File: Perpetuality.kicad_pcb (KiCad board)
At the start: 2 copper layers, 33 x 36.5 mm, 27 parts, among them J1 Conn_01x04, J2 Conn_01x01, J3 Conn_01x01, J4 Conn_01x01, U1 XIAO-nRF52840-SMD, U2 NCV8164CSN180T1G, U3 ICM-20948, U4 INA333xxDGK, U5 OPA333xxDCK, U6 ADS8866IDGS

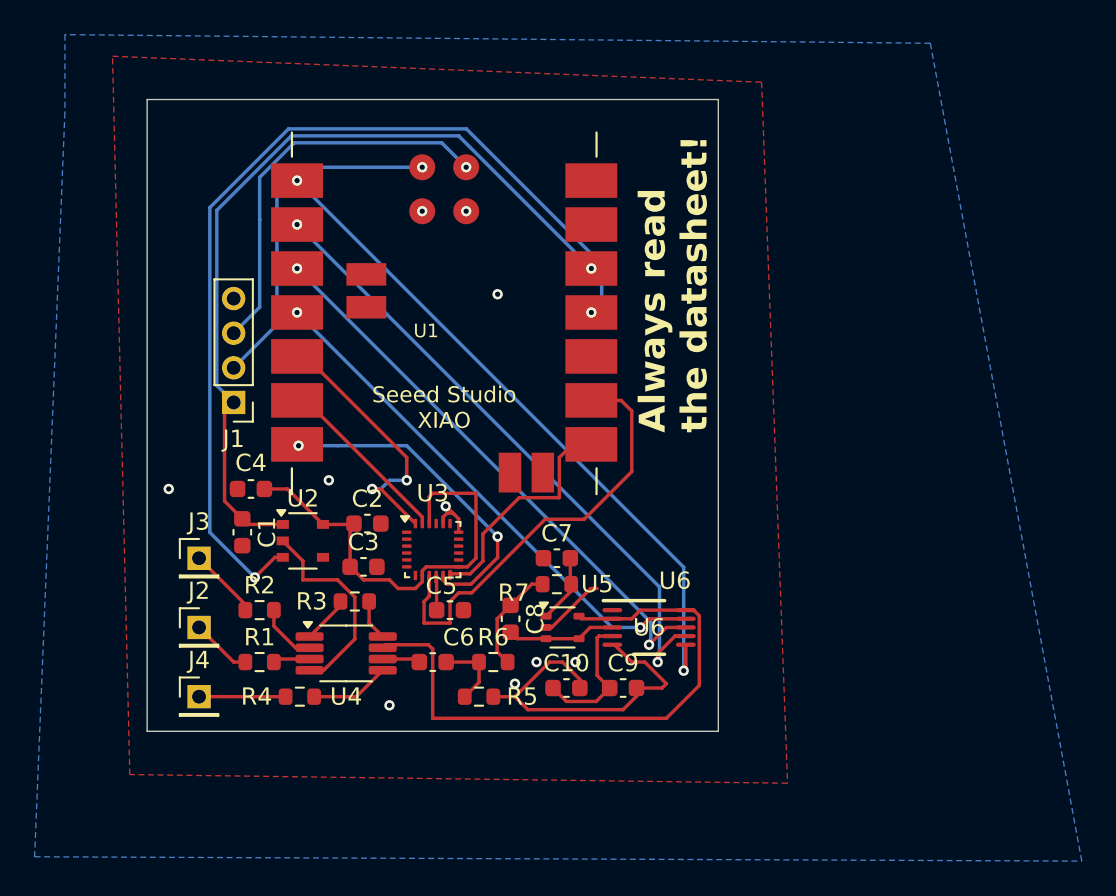
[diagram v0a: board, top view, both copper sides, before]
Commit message: newest version sent to jlc
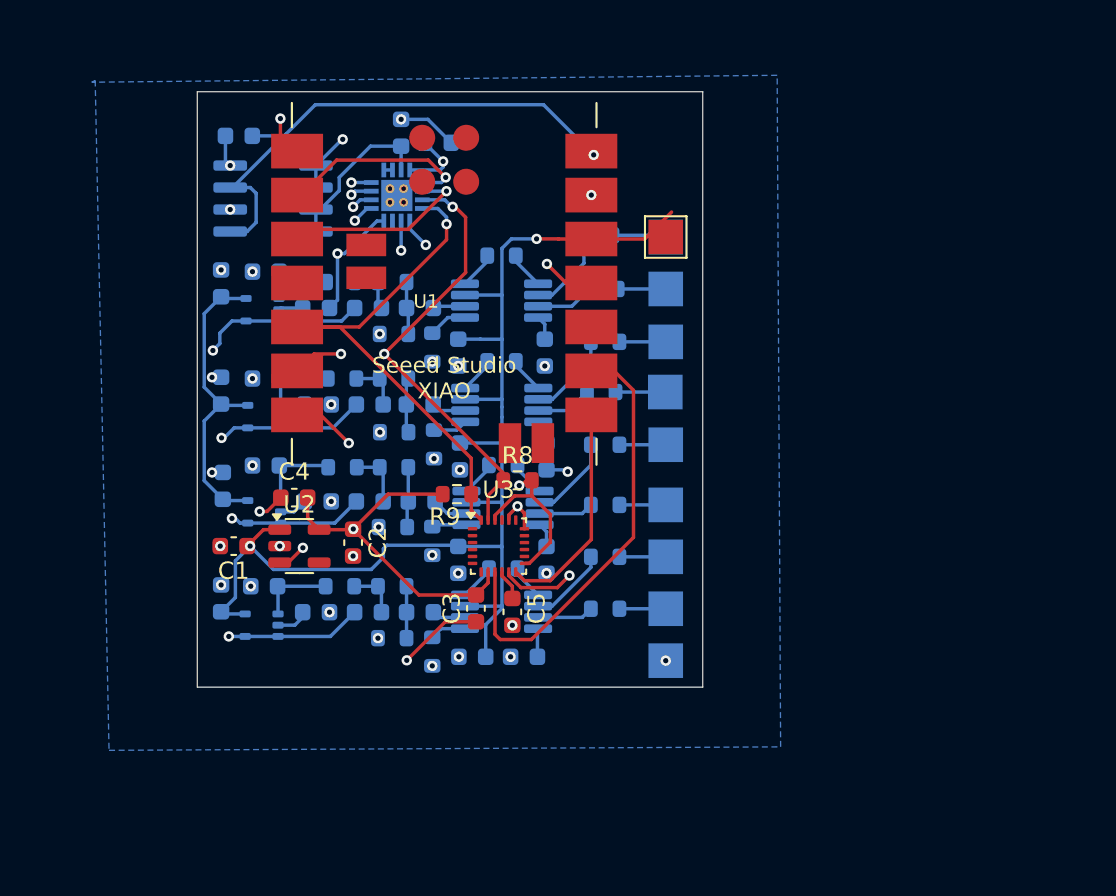
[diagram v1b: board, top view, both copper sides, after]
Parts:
- added ...: Conn_01x01, TestPoint:TestPoint_Pad_2.0x2.0mm, B.Cu at (80.5, 78.0)
- added C11: 33nF, Capacitor_SMD:C_0603_1608Metric, B.Cu at (63.4, 81.6)
- added C12: 33nF, Capacitor_SMD:C_0603_1608Metric, B.Cu at (57.4, 80.1)
- added C13: 0.1uF, Capacitor_SMD:C_0603_1608Metric, B.Cu at (60.4, 81.6)
- added C14: 0.1uF, Capacitor_SMD:C_0603_1608Metric, B.Cu at (54.8, 80.8)
- added C15: 2.2µF, Capacitor_SMD:C_0603_1608Metric, B.Cu at (55.8, 66.1)
- added C16: 1µF, Capacitor_SMD:C_0603_1608Metric, B.Cu at (66.3, 76.0)
- added C17: 0.1uF, Capacitor_SMD:C_0603_1608Metric, B.Cu at (73.5, 78.6)
- added C18: 0.1uF, Capacitor_SMD:C_0603_1608Metric, B.Cu at (68.5, 78.6)
- added C19: 33nF, Capacitor_SMD:C_0603_1608Metric, B.Cu at (57.4, 73.9)
- added C20: 33nF, Capacitor_SMD:C_0603_1608Metric, B.Cu at (63.3, 76.0)
- added C21: 0.1uF, Capacitor_SMD:C_0603_1608Metric, B.Cu at (60.3, 76.0)
- added C22: 0.1uF, Capacitor_SMD:C_0603_1608Metric, B.Cu at (54.8, 74.6)
- added C23: 0.1uF, Capacitor_SMD:C_0603_1608Metric, B.Cu at (73.6, 90.6)
- added C24: 0.1uF, Capacitor_SMD:C_0603_1608Metric, B.Cu at (68.5, 90.6)
- added C25: 1µF, Capacitor_SMD:C_0603_1608Metric, B.Cu at (66.4, 87.2)
- added C26: 33nF, Capacitor_SMD:C_0603_1608Metric, B.Cu at (63.4, 87.2)
- added C27: 33nF, Capacitor_SMD:C_0603_1608Metric, B.Cu at (57.4, 85.1)
- added C28: 0.1uF, Capacitor_SMD:C_0603_1608Metric, B.Cu at (60.4, 87.2)
- added C29: 0.1uF, Capacitor_SMD:C_0603_1608Metric, B.Cu at (54.9, 86.3)
- added C30: 0.1uF, Capacitor_SMD:C_0603_1608Metric, B.Cu at (72.3, 96.2)
- added C31: 0.1uF, Capacitor_SMD:C_0603_1608Metric, B.Cu at (69.3, 96.2)
- added C32: 1µF, Capacitor_SMD:C_0603_1608Metric, B.Cu at (66.3, 93.6)
- added C33: 33nF, Capacitor_SMD:C_0603_1608Metric, B.Cu at (63.3, 93.6)
- added C34: 33nF, Capacitor_SMD:C_0603_1608Metric, B.Cu at (57.3, 92.1)
- added C35: 0.1uF, Capacitor_SMD:C_0603_1608Metric, B.Cu at (60.3, 93.6)
- added C36: 0.1uF, Capacitor_SMD:C_0603_1608Metric, B.Cu at (54.8, 92.8)
- added EMG4+: Conn_01x01, TestPoint:TestPoint_Pad_2.0x2.0mm, B.Cu at (80.4, 80.9)
- added J10: Conn_01x01, TestPoint:TestPoint_Pad_2.0x2.0mm, B.Cu at (80.5, 90.4)
- added J7: Conn_01x01, TestPoint:TestPoint_Pad_2.0x2.0mm, B.Cu at (80.5, 87.4)
- added J9: Conn_01x01, TestPoint:TestPoint_Pad_2.0x2.0mm, B.Cu at (80.5, 93.4)
- added R10: 470Ω, Resistor_SMD:R_0603_1608Metric, B.Cu at (71.0, 73.0)
- added R11: 47kΩ, Resistor_SMD:R_0603_1608Metric, B.Cu at (76.9, 74.9)
- added R12: 47kΩ, Resistor_SMD:R_0603_1608Metric, B.Cu at (76.6, 71.8)
- added R13: 47kΩ, Resistor_SMD:R_0603_1608Metric, B.Cu at (67.0, 78.3)
- added R14: 15.9kΩ, Resistor_SMD:R_0603_1608Metric, B.Cu at (64.8, 77.5)
- added R15: 10kΩ, Resistor_SMD:R_0603_1608Metric, B.Cu at (64.7, 74.5)
- added R16: 10kΩ, Resistor_SMD:R_0603_1608Metric, B.Cu at (61.7, 74.5)
- added R17: 470Ω, Resistor_SMD:R_0603_1608Metric, B.Cu at (71.1, 85.1)
- added R18: 47kΩ, Resistor_SMD:R_0603_1608Metric, B.Cu at (77.0, 87.4)
- added R19: 47kΩ, Resistor_SMD:R_0603_1608Metric, B.Cu at (77.0, 83.9)
- added R20: 47kΩ, Resistor_SMD:R_0603_1608Metric, B.Cu at (67.0, 89.5)
- added R21: 15.9kΩ, Resistor_SMD:R_0603_1608Metric, B.Cu at (64.7, 88.7)
- added R22: 10kΩ, Resistor_SMD:R_0603_1608Metric, B.Cu at (64.8, 85.2)
- added R23: 10kΩ, Resistor_SMD:R_0603_1608Metric, B.Cu at (61.8, 85.2)
- added R24: 470Ω, Resistor_SMD:R_0603_1608Metric, B.Cu at (71.1, 91.1)
- added R25: 47kΩ, Resistor_SMD:R_0603_1608Metric, B.Cu at (77.0, 93.4)
- added R26: 47kΩ, Resistor_SMD:R_0603_1608Metric, B.Cu at (77.0, 90.4)
- added R27: 47kΩ, Resistor_SMD:R_0603_1608Metric, B.Cu at (67.0, 95.9)
- added R28: 15.9kΩ, Resistor_SMD:R_0603_1608Metric, B.Cu at (64.7, 95.1)
- added R29: 10kΩ, Resistor_SMD:R_0603_1608Metric, B.Cu at (64.7, 92.1)
- added R30: 10kΩ, Resistor_SMD:R_0603_1608Metric, B.Cu at (61.6, 92.1)
- added R8: 3kΩ, Resistor_SMD:R_0603_1608Metric, F.Cu at (71.9, 86.0)
- added R9: 3kΩ, Resistor_SMD:R_0603_1608Metric, F.Cu at (68.4, 86.8)
- added REF: Conn_01x01, TestPoint:TestPoint_Pad_2.0x2.0mm, B.Cu at (80.5, 83.9)
- added U10: INA333xxDGK, Package_SO:VSSOP-8_3x3mm_P0.65mm, B.Cu at (71.1, 87.6)
- added U11: OPA333xxDCK, Package_TO_SOT_SMD:SOT-353_SC-70-5, B.Cu at (57.3, 87.8)
- added U12: INA333xxDGK, Package_SO:VSSOP-8_3x3mm_P0.65mm, B.Cu at (71.0, 93.6)
- added U13: OPA333xxDCK, Package_TO_SOT_SMD:SOT-353_SC-70-5, B.Cu at (57.1, 94.4)
- added U7: ADS7924IRTER, perpetuality_footprints:RTE16_1P7X1P7, B.Cu at (64.9, 69.5)
- added U8: MCP1501-33xSN, Package_SO:SOIC-8_3.9x4.9mm_P1.27mm, B.Cu at (57.8, 69.7)
- added U9: OPA333xxDCK, Package_TO_SOT_SMD:SOT-353_SC-70-5, B.Cu at (57.2, 76.1)
- C10: value 0.1µF -> 1µF; moved to B.Cu
- C6: value 1µF -> 0.1uF; moved to B.Cu
- C7: value 33nF -> 0.1uF; moved to B.Cu
- C8: value 33nF -> 1µF; moved to B.Cu
- C9, R2, R4, R5, R6, R7, U4, U5: moved to B.Cu
- EMG1+: renamed from J2; footprint Connector_PinHeader_2.00mm:PinHeader_1x01_P2.00mm_Vertical -> TestPoint:TestPoint_Pad_2.0x2.0mm; moved to B.Cu
- EMG1-: renamed from J3; footprint Connector_PinHeader_2.00mm:PinHeader_1x01_P2.00mm_Vertical -> TestPoint:TestPoint_Pad_2.0x2.0mm; moved to B.Cu
- J1: footprint Connector_PinHeader_2.00mm:PinHeader_1x04_P2.00mm_Vertical -> TestPoint:TestPoint_Pad_2.0x2.0mm
- J4: footprint Connector_PinHeader_2.00mm:PinHeader_1x01_P2.00mm_Vertical -> TestPoint:TestPoint_Pad_2.0x2.0mm; moved to B.Cu
- R1: value 47kΩ -> 470Ω; moved to B.Cu
- R3: value 470Ω -> 47kΩ; moved to B.Cu
- U2: footprint Package_SO:TSOP-5_1.65x3.05mm_P0.95mm -> Package_TO_SOT_SMD:TSOT-23-5
- U6: value ADS8866IDGS -> INA333xxDGK; footprint perpetuality_footprints:DGS0010A_L -> Package_SO:VSSOP-8_3x3mm_P0.65mm; moved to B.Cu
- moved C10 33.5 mm to (65.2, 65.9), turned to 90 degrees
- moved EMG1+ 33.3 mm to (80.5, 74.9), turned to 180 degrees
- moved C9 33.3 mm to (67.3, 66.5)
- moved EMG1- 32.7 mm to (80.5, 71.9), turned to 180 degrees
- moved J4 27.0 mm to (80.5, 96.4), turned to 180 degrees
- moved J1 26.7 mm to (80.5, 71.9)
- moved R2 23.4 mm to (76.7, 80.9), turned to 180 degrees
- moved R1 22.3 mm to (71.0, 79.1)
- moved U5 21.1 mm to (57.3, 82.3), turned to 180 degrees
- moved R3 20.8 mm to (77.0, 78.0)
- moved U6 20.7 mm to (71.0, 75.6), turned to 180 degrees
- moved R6 17.4 mm to (64.8, 80.1), turned to 180 degrees
- moved R7 17.2 mm to (61.8, 80.1), turned to 180 degrees
- moved U4 16.9 mm to (71.0, 81.6), turned to 180 degrees
- moved R4 16.5 mm to (67.1, 83.9), turned to 90 degrees
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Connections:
- net Net-(J4-Pin_1) renamed REF
- C1 pad 2: GND -> GNDD
- C10 pad 1: Net-(U6-AINN) -> VREF
- C10 pad 2: GND -> GNDD
- C2 pad 2: GND -> GNDD
- C3 pad 2: GND -> GNDD
- C4 pad 2: GND -> GNDD
- C5 pad 2: GND -> GNDD
- C6 pad 1: Amplified Signal -> Net-(U4-V-)
- C6 pad 2: High-pass Signal -> GND
- C7 pad 1: GND -> 3V3
- C7 pad 2: Net-(U5-+) -> GND
- C8 pad 1: Net-(C8-Pad1) -> /EMG2/Amplified_Signal
- C8 pad 2: Filtered Signal -> /EMG2/High-pass_Signal
- C9 pad 1: Net-(U6-AINN) -> 1V8
- C9 pad 2: GND -> GNDD
- EMG1+ pad 1: Net-(J2-Pin_1) -> E1+
- EMG1- pad 1: Net-(J3-Pin_1) -> E1-
- R1 pad 1: Net-(J2-Pin_1) -> Net-(R1-Pad1)
- R1 pad 2: Net-(U4-+) -> Net-(R1-Pad2)
- R2 pad 1: Net-(J3-Pin_1) -> E2+
- R2 pad 2: Net-(U4--) -> Net-(U4-+)
- R3 pad 1: Net-(R3-Pad1) -> E2-
- R3 pad 2: Net-(R3-Pad2) -> Net-(U4--)
- R5 pad 2: High-pass Signal -> /EMG2/High-pass_Signal
- R6 pad 1: High-pass Signal -> /EMG2/High-pass_Signal
- R6 pad 2: Net-(C8-Pad1) -> Net-(C11-Pad1)
- R7 pad 1: Net-(C8-Pad1) -> Net-(C11-Pad1)
- U1 pad 1: CONVST -> A0
- U1 pad 13: GND -> GNDD
- U1 pad 14: unconnected-(U1-5V-Pad14) -> 5V
- U1 pad 15: SWDIO -> (no net)
- U1 pad 16: SWCLK -> (no net)
- U1 pad 17: unconnected-(U1-RESET-Pad17) -> (no net)
- U1 pad 18: GND -> (no net)
- U1 pad 19: unconnected-(U1-NFC1-Pad19) -> (no net)
- U1 pad 2: DOUT -> *RESET
- U1 pad 20: unconnected-(U1-NFC2-Pad20) -> (no net)
- U1 pad 21: unconnected-(U1-BAT-Pad21) -> (no net)
- U1 pad 22: Net-(U1-GND-Pad22) -> (no net)
- U1 pad 3: SCLK -> *INT
- U1 pad 4: DIN -> unconnected-(U1-P0.29_A3_D3-Pad4)
- U2 pad 2: GND -> GNDD
- U3 pad 18: GND -> GNDD
- U3 pad 20: GND -> GNDD
- U4 pad 1: Net-(R3-Pad2) -> Net-(R1-Pad2)
- U4 pad 4: GND -> Net-(U4-V-)
- U4 pad 6: Amplified Signal -> /EMG2/Amplified_Signal
- U4 pad 7: +3.3V -> 3V3
- U4 pad 8: Net-(R3-Pad1) -> Net-(R1-Pad1)
- U5 pad 2: GND -> Net-(U5-V-)
- U5 pad 3: Filtered Signal -> /EMG2/EMG_OUT
- U5 pad 4: Filtered Signal -> /EMG2/EMG_OUT
- U5 pad 5: +3.3V -> 3V3
- U6 pad 1: +5V -> Net-(R10-Pad2)
- U6 pad 2: +3.3V -> Net-(U6--)
- U6 pad 3: Filtered Signal -> Net-(U6-+)
- U6 pad 4: Net-(U6-AINN) -> Net-(U6-V-)
- U6 pad 5: GND -> Net-(U6-Ref)
- U6 pad 6: CONVST -> /EMG1/Amplified_Signal
- U6 pad 7: DOUT -> 3V3
- U6 pad 8: SCLK -> Net-(R10-Pad1)
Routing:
- net 3V3: track 47.9 -> 90.4 mm, vias 1 -> 2
- net CONVST: track 39.1 -> 0.00 mm, vias 2 -> 0
- net DOUT: track 36.5 -> 0.00 mm, vias 2 -> 0
- net /EMG4/EMG_OUT: track 0.00 -> 36.1 mm, vias 0 -> 2
- net +3.3V: track 34.6 -> 0.00 mm
- net SCLK: track 32.9 -> 0.00 mm, vias 2 -> 0
- net GND: track 39.6 -> 8.06 mm, vias 9 -> 24
- net 5V: track 0.00 -> 31.2 mm, vias 0 -> 1
- net DIN: track 30.2 -> 0.00 mm, vias 2 -> 0
- net /EMG3/EMG_OUT: track 0.00 -> 30.0 mm, vias 0 -> 2
- net /EMG2/EMG_OUT: track 0.00 -> 27.4 mm, vias 0 -> 2
- net EN: track 55.3 -> 28.2 mm
- net REF: track 5.00 -> 31.3 mm, vias 0 -> 5
- net /EMG1/EMG_OUT: track 0.00 -> 24.7 mm, vias 0 -> 2
- net SWCLK: track 23.0 -> 0.00 mm, vias 1 -> 0
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- added copper zone on In1.Cu, net 1V8
- added copper zone on B.Cu, net 3V3
- added copper zone on In4.Cu, net GND
- added copper zone on In2.Cu, net GNDD
- removed copper zone on B.Cu, net GND
- removed copper zone on F.Cu, net GND
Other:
- board size 33 x 36.5 mm -> 29.2 x 34.4 mm
- copper layers 2 -> 6
- board text added: "${REFERENCE}"
- board text added: "Component"
- board text added: "Directly Below"
- board text added: "KEEPOUT"
- board text added: "No Copper"
- board text removed: "Always read the datasheet!"
